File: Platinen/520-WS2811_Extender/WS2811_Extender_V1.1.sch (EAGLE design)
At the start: 26 parts, among them IC1 ULN2003AN, J1 Out2, J2 Out3, J4 Out1, U2R TINY45-20-DIP, U3H WS2811 SOT-8

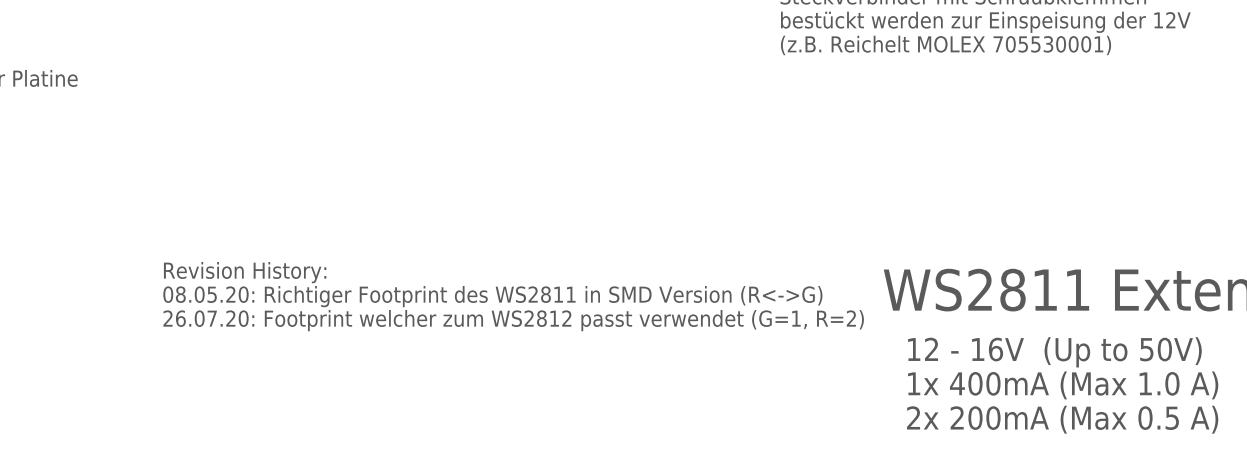
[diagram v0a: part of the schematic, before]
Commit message: Ver.:1.1
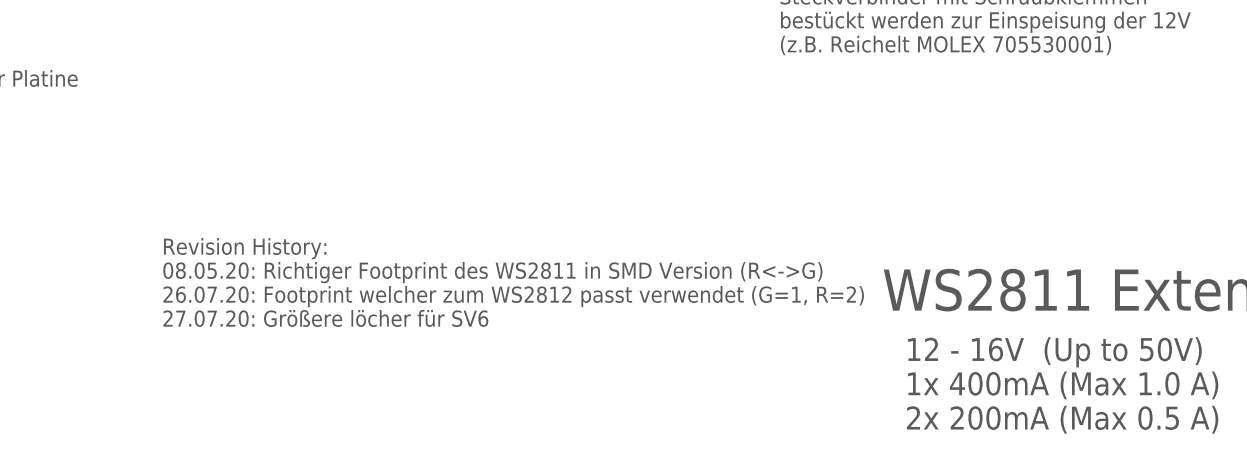
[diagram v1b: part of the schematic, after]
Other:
- note added: "Revision History: 08.05.20: Richtiger Footprint des WS2811 in SMD Version (R<->G) 26.07.20: Footprint welcher zum WS2812 passt verwendet (G=1, R=2) 27.07.20: Größere löcher für SV6"
- note removed: "Revision History: 08.05.20: Richtiger Footprint des WS2811 in SMD Version (R<->G) 26.07.20: Footprint welcher zum WS2812 passt verwendet (G=1, R=2)"
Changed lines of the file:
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@@
 <text x="82.55" y="16.51" size="1.778" layer="97">Revision History:
 08.05.20: Richtiger Footprint des WS2811 in SMD Version (R&lt;-&gt;G)
-26.07.20: Footprint welcher zum WS2812 passt verwendet (G=1, R=2)</text>
+26.07.20: Footprint welcher zum WS2812 passt verwendet (G=1, R=2)
+27.07.20: Größere löcher für SV6</text>
 </plain>
 <instances>
